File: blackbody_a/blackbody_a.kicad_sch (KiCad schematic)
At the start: 26 parts, among them J1 CarPowerConnector, SW4 SW_SPDT, SW5 SW_Push, SW6 Reset, U3 STM32L431CBTx, Y1 8M

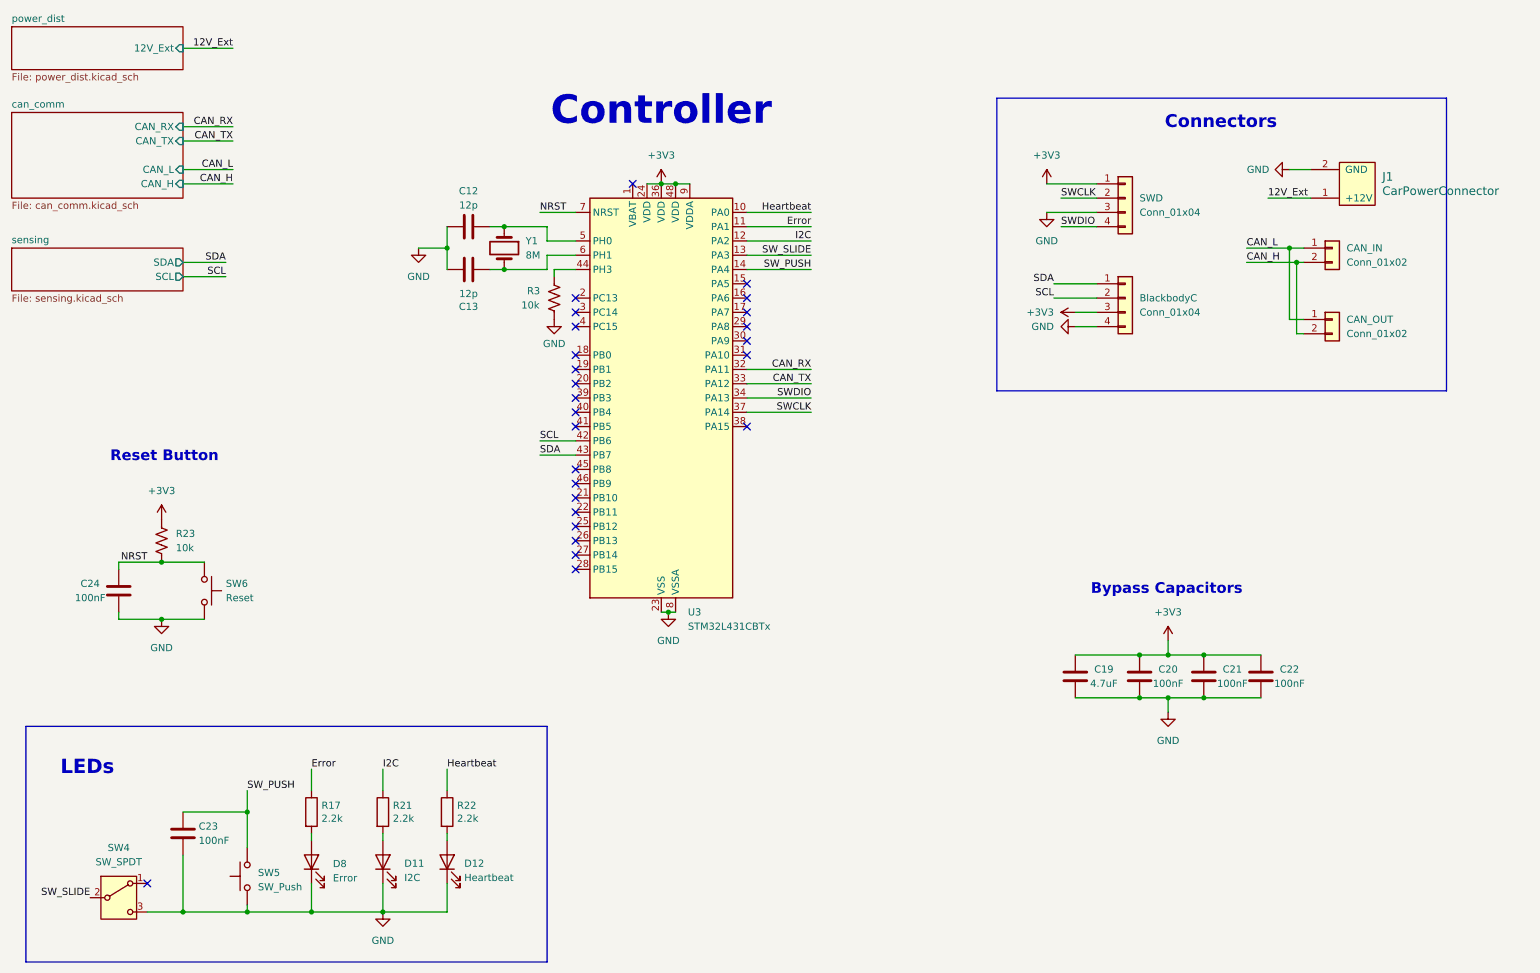
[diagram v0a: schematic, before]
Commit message: layout iteration 1
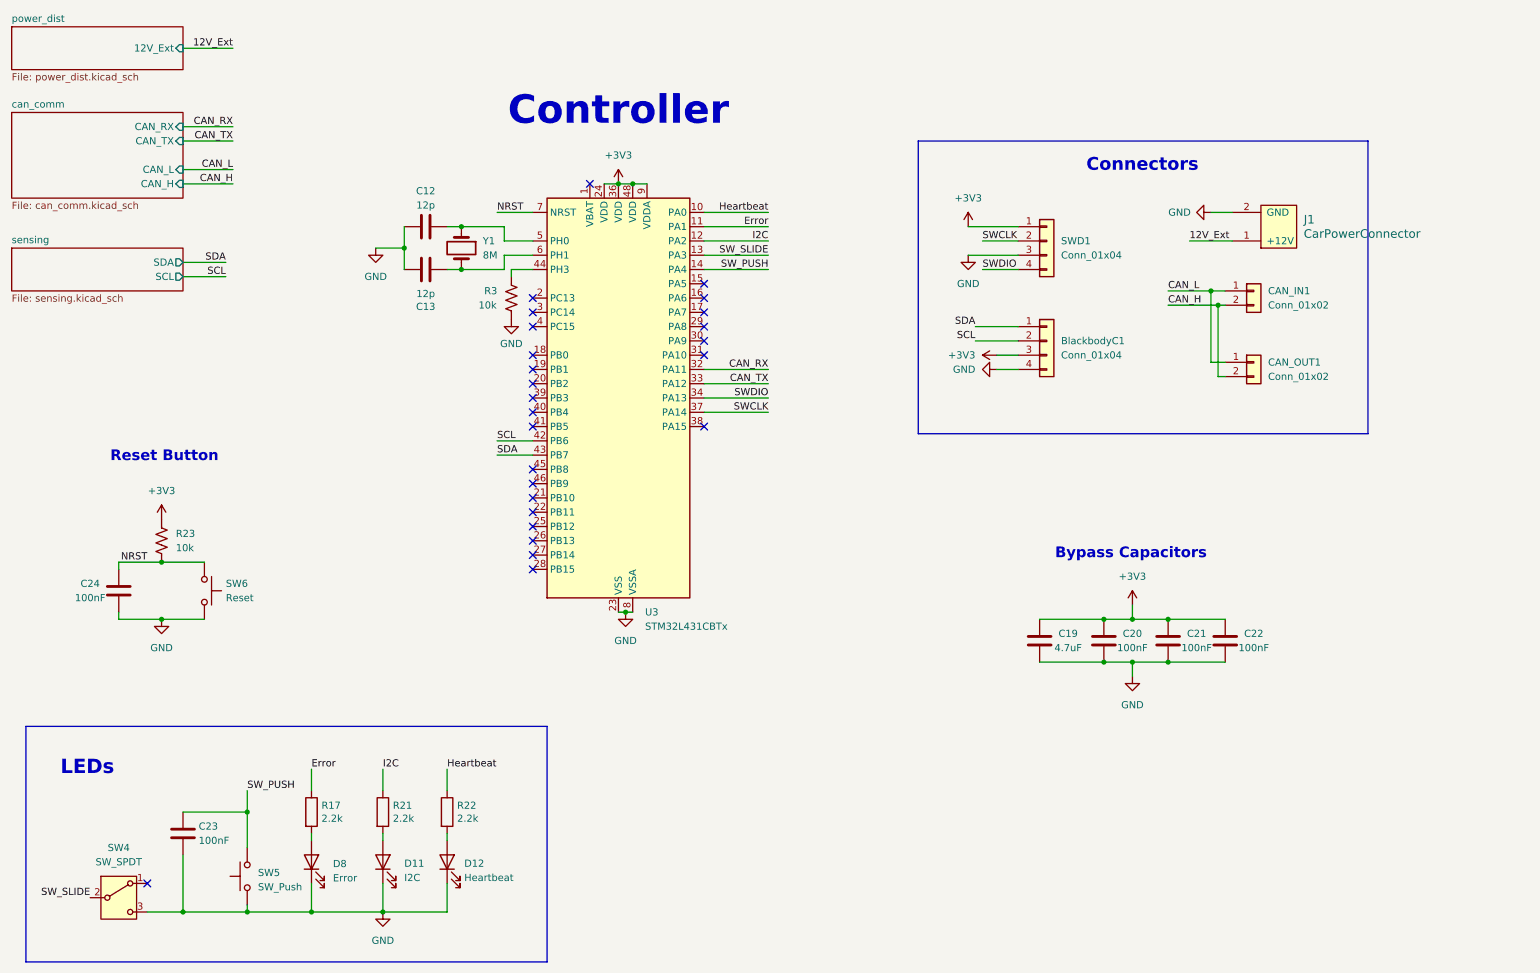
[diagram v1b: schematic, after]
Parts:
- BlackbodyC1: renamed from BlackbodyC; footprint (none) -> blackbodies:MOLEX_1053091104
- C12, C13, C19, C20, C21, C22, C24: footprint (none) -> Capacitor_SMD:C_0805_2012Metric
- CAN_IN1: renamed from CAN_IN; footprint (none) -> Connector_PinHeader_2.54mm:PinHeader_1x02_P2.54mm_Vertical
- CAN_OUT1: renamed from CAN_OUT; footprint (none) -> Connector_PinHeader_2.54mm:PinHeader_1x02_P2.54mm_Vertical
- J1: footprint (none) -> UTSVT_Connectors:Molex_MicroFit3.0_1x2xP3.00mm_PolarizingPeg_Vertical
- R23, R3: footprint (none) -> Resistor_SMD:R_0805_2012Metric
- SW4: footprint (none) -> Button_Switch_SMD:SW_DIP_SPSTx01_Slide_6.7x4.1mm_W6.73mm_P2.54mm_LowProfile_JPin
- SW6: footprint (none) -> Button_Switch_SMD:SW_SPST_B3SL-1002P
- SWD1: renamed from SWD; footprint (none) -> Connector_PinHeader_2.54mm:PinHeader_1x04_P2.54mm_Vertical
- Y1: footprint (none) -> UTSVT_Special:ABM3
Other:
- moved on the sheet: BlackbodyC1, C12, C13, C19, C20, C21, C22, CAN_IN1, CAN_OUT1, J1, R3, SWD1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
